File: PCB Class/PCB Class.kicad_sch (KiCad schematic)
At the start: 0 parts

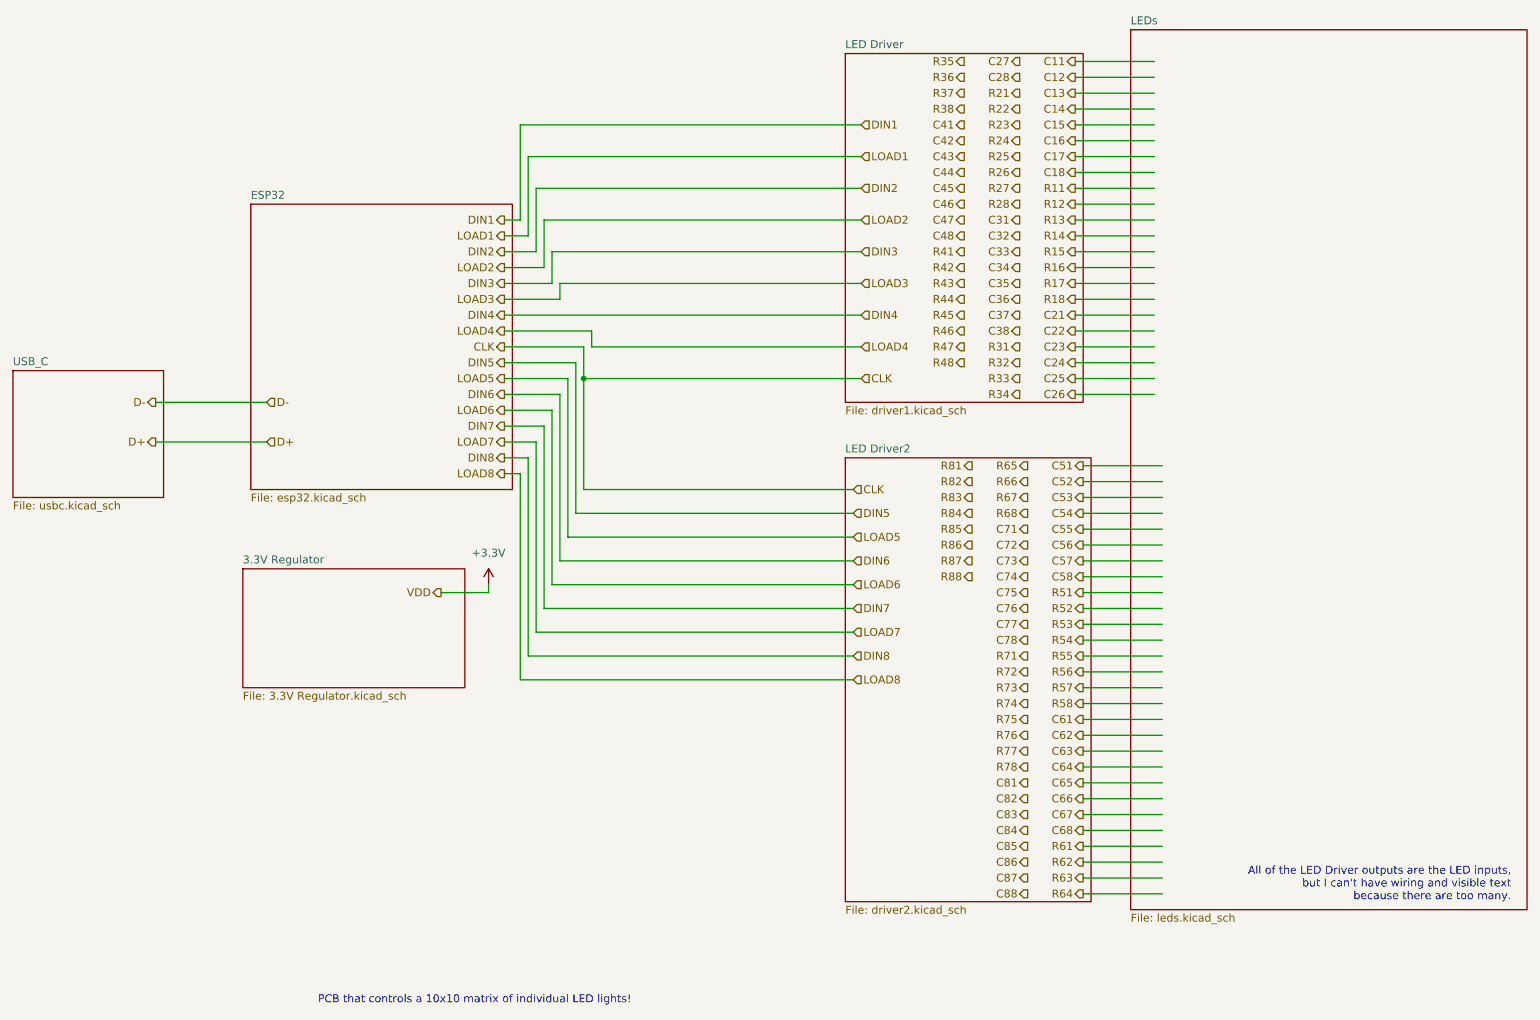
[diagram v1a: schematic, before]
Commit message: Layout
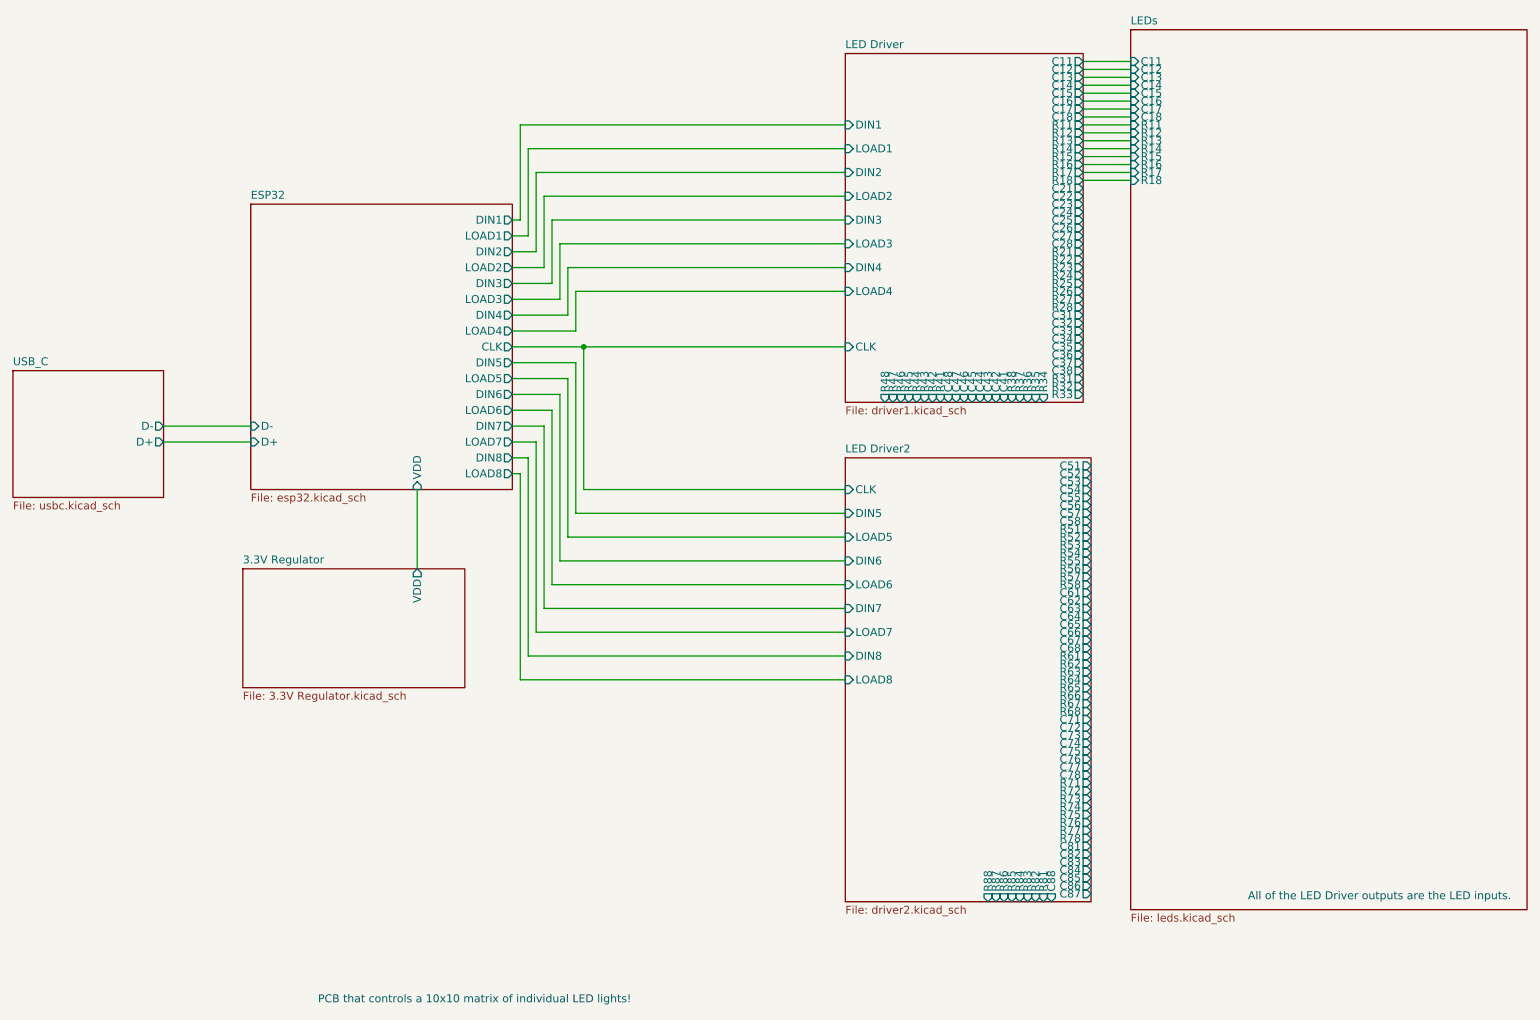
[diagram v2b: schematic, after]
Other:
- sheet 3.3V Regulator ports: added VDD; removed none
- sheet ESP32 ports: added CLK, D+, D-, DIN1, DIN2, DIN3, DIN4, DIN5, DIN6, DIN7, DIN8, LOAD1, LOAD2, LOAD3, LOAD4, LOAD5, LOAD6, LOAD7, LOAD8, VDD; removed none
- sheet LED Driver ports: added C11, C12, C13, C14, C15, C16, C17, C18, C21, C22, C23, C24, C25, C26, C27, C28, C31, C32, C33, C34, C35, C36, C37, C38, C41, C42, C43, C44, C45, C46, C47, C48, CLK, DIN1, DIN2, DIN3, DIN4, LOAD1, LOAD2, LOAD3, LOAD4, R11, R12, R13, R14, R15, R16, R17, R18, R21, R22, R23, R24, R25, R26, R27, R28, R31, R32, R33, R34, R35, R36, R37, R38, R41, R42, R43, R44, R45, R46, R47, R48; removed none
- sheet LED Driver2 ports: added C51, C52, C53, C54, C55, C56, C57, C58, C61, C62, C63, C64, C65, C66, C67, C68, C71, C72, C73, C74, C75, C76, C77, C78, C81, C82, C83, C84, C85, C86, C87, C88, CLK, DIN5, DIN6, DIN7, DIN8, LOAD5, LOAD6, LOAD7, LOAD8, R51, R52, R53, R54, R55, R56, R57, R58, R61, R62, R63, R64, R65, R66, R67, R68, R71, R72, R73, R74, R75, R76, R77, R78, R81, R82, R83, R84, R85, R86, R87, R88; removed none
- sheet LEDs ports: added C11, C12, C13, C14, C15, C16, C17, C18, R11, R12, R13, R14, R15, R16, R17, R18; removed none
- sheet USB_C ports: added D+, D-; removed none
- note added: "All of the LED Driver outputs are the LED inputs."
- note removed: "All of the LED Driver outputs are the LED inputs, but I can't have wiring and visible text because there are too many."
